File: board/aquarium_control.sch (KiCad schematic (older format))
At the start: 22 parts, among them J1 Barrel_Jack, J1 RPi, J2 Day_Light, J3 Night_Light, J4 Temp_Sensor, J5 LCD, J6 SPI, U1 AP1507, U2 VO14642, U3 VO14642

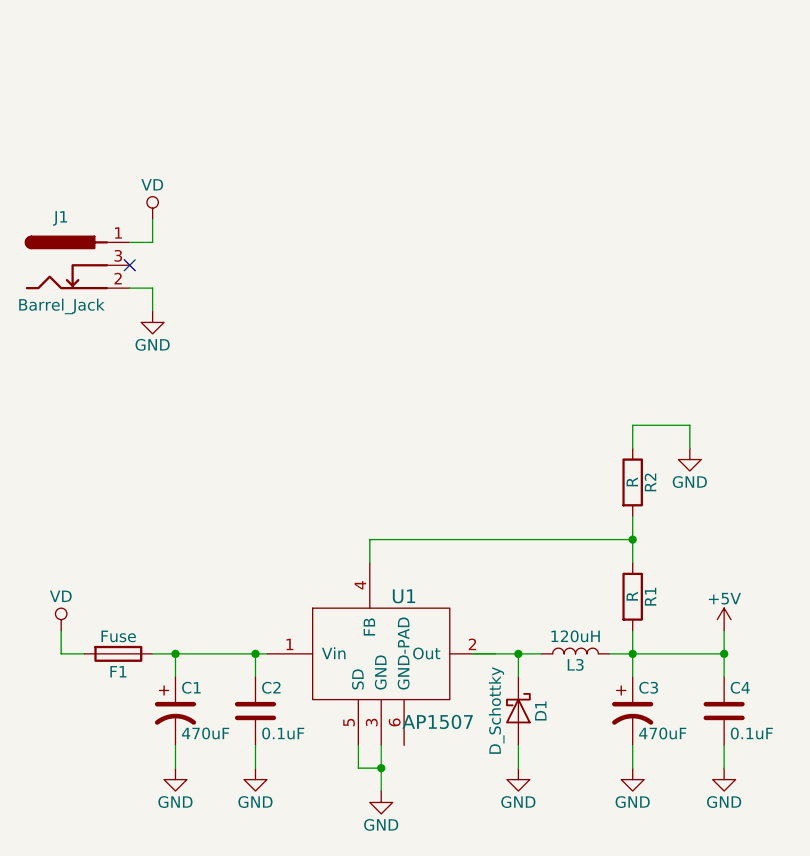
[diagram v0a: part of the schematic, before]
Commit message: Updates to the board
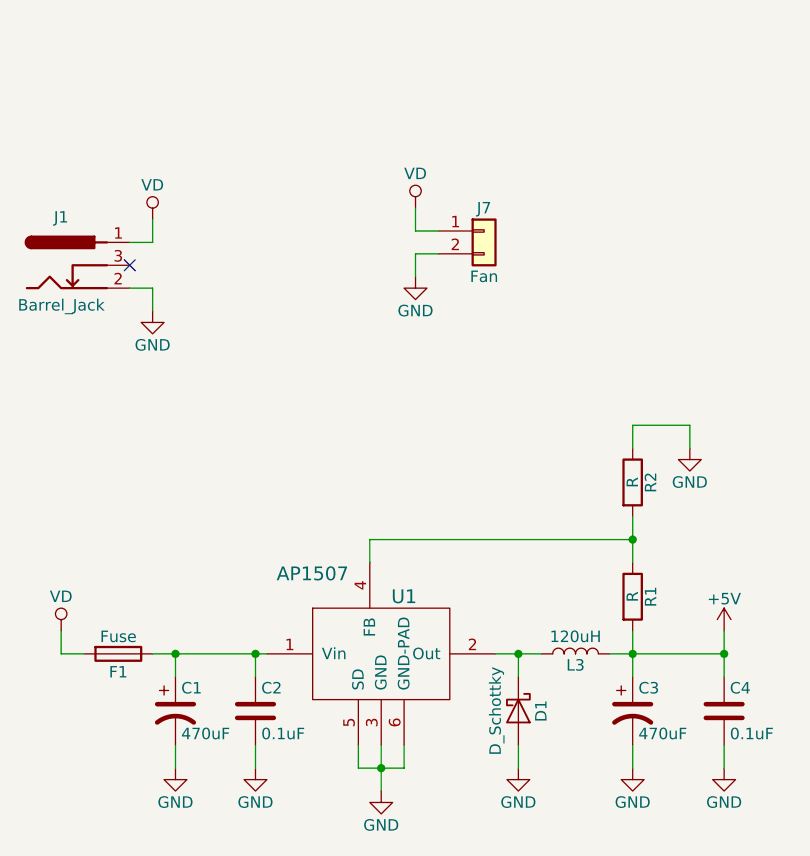
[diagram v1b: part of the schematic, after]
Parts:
- added J7: Fan, Pin_Headers:Pin_Header_Straight_1x02_Pitch2.54mm, symbol Conn_01x02
- U1: footprint (none) -> nebrius-regulator:AP1507
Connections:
- net GND: now also U1.6 (GND-PAD), J7.2 (Pin_2)
- net VD: now also J7.1 (Pin_1)
- net at D1.1 (K), L3.1: now also U1.2 (Out)
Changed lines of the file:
@@
 	2800 4650 2800 4750
 Wire Wire Line
-	2800 4750 2900 4750
+	2800 4750 3000 4750
 Connection ~ 2900 4750
 $Comp
@@
 $EndComp
 Wire Wire Line
-	3300 4250 3600 4250
-Wire Wire Line
 	3500 4250 3500 4350
 $Comp
@@
 	6600 4500 6150 4500
 $Comp
-L AP1507 U1
-U 1 1 5A189BEF
-P 2950 4100
-F 0 "U1" H 3000 4200 60  0000 C CNN
-F 1 "AP1507" H 3150 3650 60  0000 C CNN
-F 2 "" H 2950 4100 60  0001 C CNN
-F 3 "" H 2950 4100 60  0001 C CNN
-	1    2950 4100
-	1    0    0    -1
-$EndComp
-$Comp
 L VO14642 U3
 U 1 1 5A189F0E
@@
 	1    0    0    -1
 $EndComp
+$Comp
+L AP1507 U1
+U 1 1 5A18C3F5
+P 2950 4100
+F 0 "U1" H 3000 4200 60  0000 C CNN
+F 1 "AP1507" H 2600 4300 60  0000 C CNN
+F 2 "nebrius-regulator:AP1507" H 2950 4100 60  0001 C CNN
+F 3 "" H 2950 4100 60  0001 C CNN
+	1    2950 4100
+	1    0    0    -1
+$EndComp
+Wire Wire Line
+	3000 4750 3000 4650
+$Comp
+L Conn_01x02 J7
+U 1 1 5A18C694
+P 3350 2400
+F 0 "J7" H 3350 2500 50  0000 C CNN
+F 1 "Fan" H 3350 2200 50  0000 C CNN
+F 2 "Pin_Headers:Pin_Header_Straight_1x02_Pitch2.54mm" H 3350 2400 50  0001 C CNN
+F 3 "" H 3350 2400 50  0001 C CNN
+	1    3350 2400
+	1    0    0    -1
+$EndComp
+$Comp
+L GND #PWR?
+U 1 1 5A18C7C8
+P 3050 2600
+F 0 "#PWR?" H 3050 2350 50  0001 C CNN
+F 1 "GND" H 3050 2450 50  0000 C CNN
+F 2 "" H 3050 2600 50  0001 C CNN
+F 3 "" H 3050 2600 50  0001 C CNN
+	1    3050 2600
+	1    0    0    -1
+$EndComp
+$Comp
+L VD #PWR?
+U 1 1 5A18C838
+P 3050 2300
+F 0 "#PWR?" H 3050 2150 50  0001 C CNN
+F 1 "VD" H 3050 2450 50  0000 C CNN
+F 2 "" H 3050 2300 50  0001 C CNN
+F 3 "" H 3050 2300 50  0001 C CNN
+	1    3050 2300
+	1    0    0    -1
+$EndComp
+Wire Wire Line
+	3050 2300 3050 2400
+Wire Wire Line
+	3050 2400 3150 2400
+Wire Wire Line
+	3150 2500 3050 2500
+Wire Wire Line
+	3050 2500 3050 2600
+Wire Wire Line
+	3400 4250 3600 4250
 $EndSCHEMATC
